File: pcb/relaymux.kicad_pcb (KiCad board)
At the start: 2 copper layers, 120.4 x 100.4 mm, 60 parts, among them J1 A, J10 B4, J11 USB_C, J12 Debug, J2 A1, J3 A2, J4 A3, J5 A4, J6 B, J7 B1, J8 B2, J9 B3, K1 TQ2SA-5V, K2 TQ2SA-5V, K3 TQ2SA-5V, K4 TQ2SA-5V, K5 TQ2SA-5V, K6 TQ2SA-5V, K7 TQ2SA-5V, K8 TQ2SA-5V, SW1 Cycle, SW2 Boot/Clear, U1 STM32F042F6Px, U2 TBD62783A, U3 TPS2552D, U4 TLV70033_SOT23-5

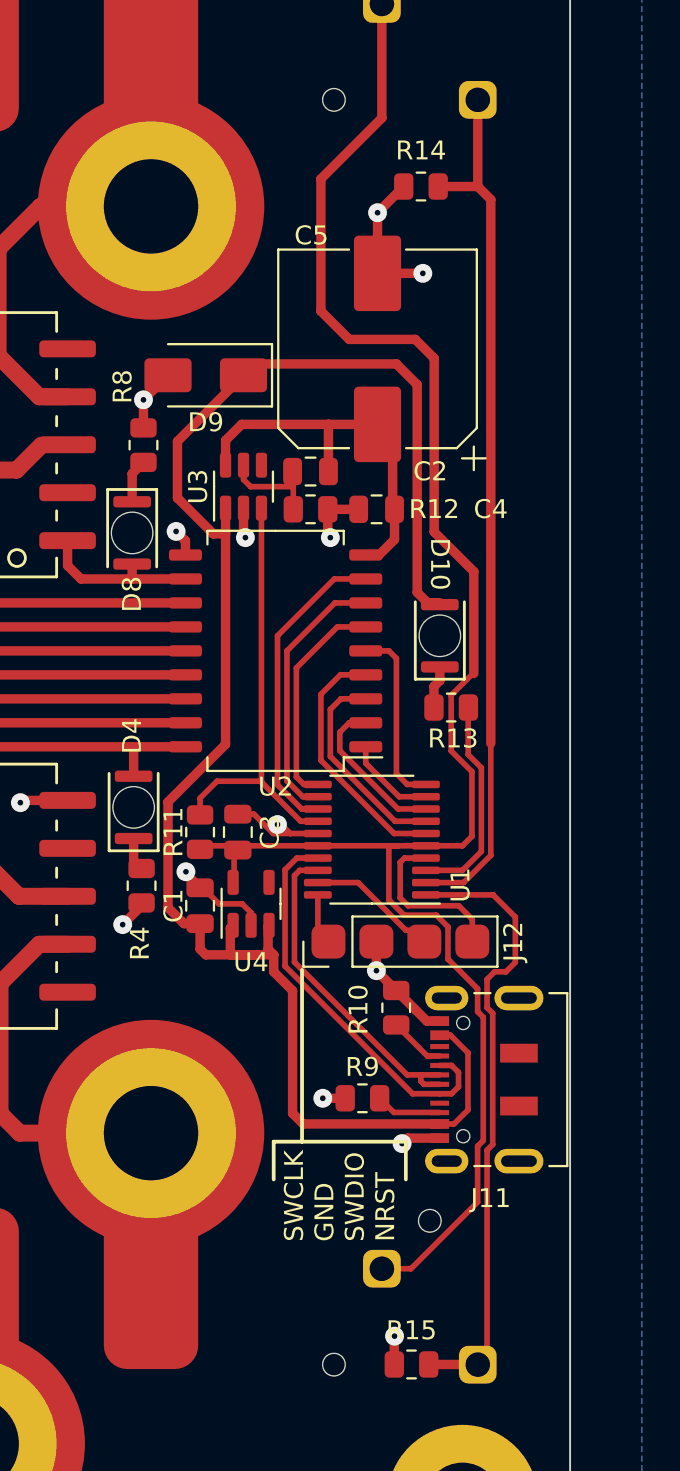
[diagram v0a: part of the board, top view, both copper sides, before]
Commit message: Add readme, BOM
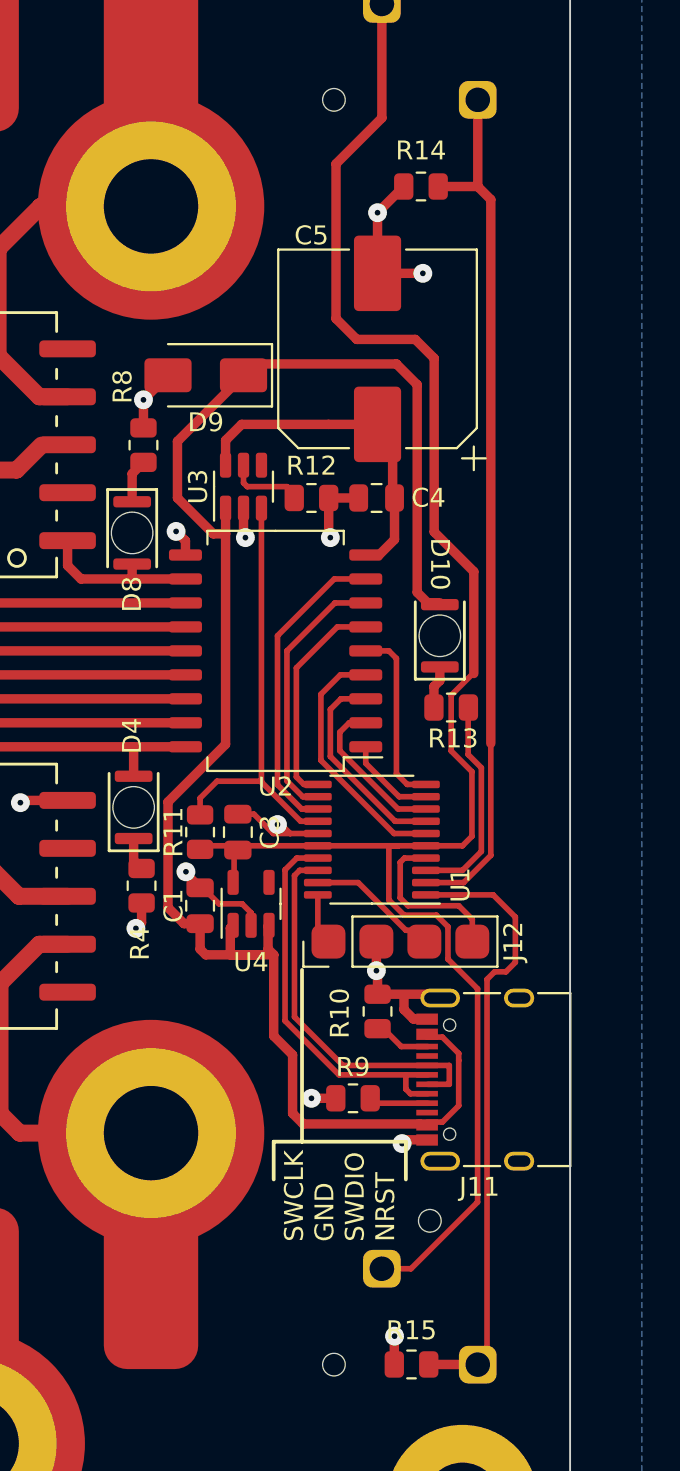
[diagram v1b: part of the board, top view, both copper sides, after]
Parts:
- removed C2: N/A, Capacitor_SMD:C_0805_2012Metric
- J11: footprint Connector_USB:USB_C_Receptacle_JAE_DX07S016JA1R1500 -> Connector_USB:USB_C_Receptacle_XKB_U262-16XN-4BVC11
- R11, R12, R14, R15: value 75k -> 68k
- moved R10 1.01 mm to (226.0, 118.6)
- moved R12 0.60 mm to (222.5, 91.4)
- moved C4 0.60 mm to (225.9, 91.4)
- moved R9 0.50 mm to (224.7, 123.2)
- moved J11 0.09 mm to (232.4, 122.2)
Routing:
- net /USB_DP: track 17.5 -> 20.2 mm
- net +5V: track 20.6 -> 18.1 mm
- net Net-(U3-ILIM): track 6.33 -> 4.08 mm
- net GND: track 73.5 -> 75.1 mm
- net +3V3: track 97.4 -> 96.3 mm
- net /VBUS: track 91.8 -> 90.9 mm
